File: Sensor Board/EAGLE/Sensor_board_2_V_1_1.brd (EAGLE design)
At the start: 15 x 65 mm, 10 parts, among them IC1 LM393N

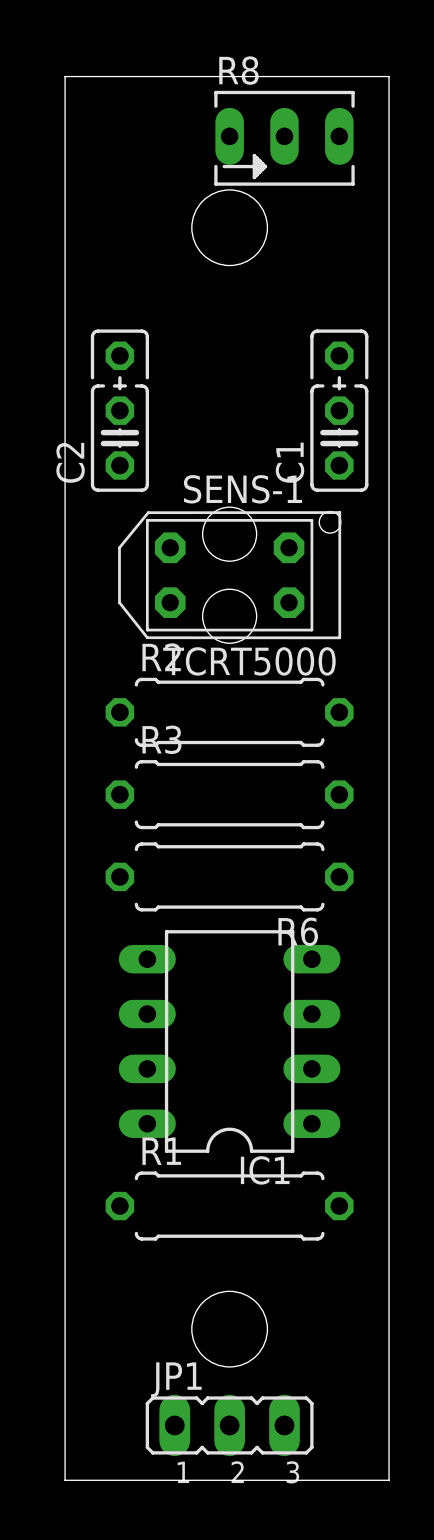
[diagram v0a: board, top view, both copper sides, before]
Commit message: Update Sensor_board_2_V_1_1.brd
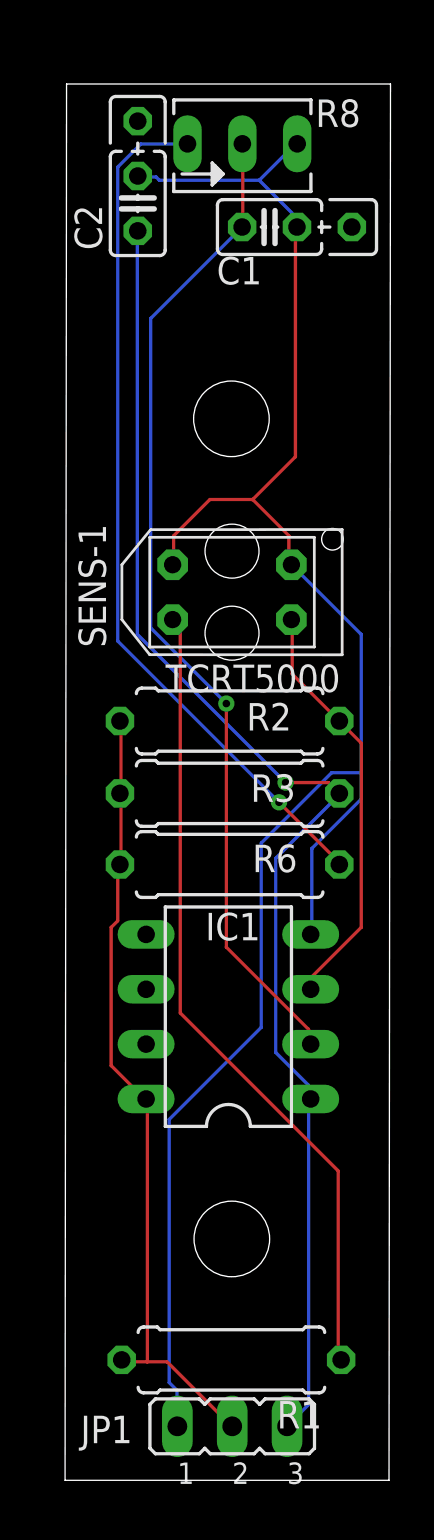
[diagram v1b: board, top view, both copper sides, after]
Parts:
- moved C2 10.9 mm to (3.37, 59.1)
- moved C1 10.3 mm to (9.47, 58.0), turned to 0 degrees
- moved R1 7.12 mm to (7.70, 5.58), turned to 180 degrees
- moved R8 1.98 mm to (8.21, 61.9)
- moved IC1 1.15 mm to (7.56, 21.5)
- moved SENS-1 0.79 mm to (7.73, 41.1)
- moved R6 0.57 mm to (7.62, 28.5)
- moved R2 0.40 mm to (7.62, 35.2)
- moved JP1 0.13 mm to (7.74, 2.50)
- moved R3 0.06 mm to (7.62, 31.8)
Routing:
- net N$3: track 0.00 -> 88.3 mm
- net N$6: track 0.00 -> 62.8 mm, vias 0 -> 1
- net N$9: track 0.00 -> 46.5 mm, vias 0 -> 1
- net N$8: track 0.00 -> 40.2 mm, vias 0 -> 1
- net N$4: track 0.00 -> 37.5 mm
- net N$1: track 0.00 -> 37.0 mm
- net N$5: track 0.00 -> 19.4 mm
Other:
- board size 15 x 65 mm -> 15.1 x 64.7 mm
